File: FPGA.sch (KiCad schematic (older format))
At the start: 1 part

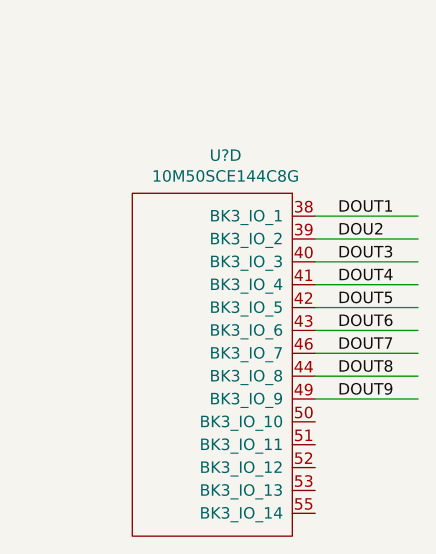
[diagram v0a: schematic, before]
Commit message: sync
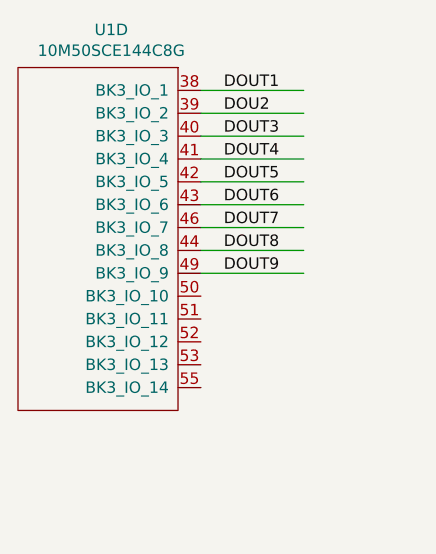
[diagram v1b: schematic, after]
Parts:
- gave numbers to parts that had none: 1
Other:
- moved on the sheet: U1D
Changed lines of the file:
@@
 $EndDescr
 $Comp
-L 10M50SCE:10M50SCE144C8G U?
+L 10M50SCE:10M50SCE144C8G U1
 U 4 1 607B5417
-P 2250 2750
-F 0 "U?" H 1942 3215 50  0000 C CNN
-F 1 "10M50SCE144C8G" H 1942 3124 50  0000 C CNN
-F 2 "10M50SCE144:QFP50P2200X2200X165-145N" H 2250 2750 50  0001 C CNN
-F 3 "" H 2250 2750 50  0001 C CNN
-	4    2250 2750
+P 1750 2200
+F 0 "U1" H 1442 2665 50  0000 C CNN
+F 1 "10M50SCE144C8G" H 1442 2574 50  0000 C CNN
+F 2 "10M50SCE144:QFP50P2200X2200X165-145N" H 1750 2200 50  0001 C CNN
+F 3 "" H 1750 2200 50  0001 C CNN
+	4    1750 2200
 	-1   0    0    -1
 $EndComp
 Wire Wire Line
-	2950 2550 3400 2550
+	2450 2000 2900 2000
 Wire Wire Line
-	2950 2650 3400 2650
+	2450 2100 2900 2100
 Wire Wire Line
-	2950 2750 3400 2750
+	2450 2200 2900 2200
 Wire Wire Line
-	2950 2850 3400 2850
+	2450 2300 2900 2300
 Wire Wire Line
-	2950 2950 3400 2950
+	2450 2400 2900 2400
 Wire Wire Line
-	2950 3050 3400 3050
+	2450 2500 2900 2500
 Wire Wire Line
-	2950 3150 3400 3150
+	2450 2600 2900 2600
 Wire Wire Line
-	2950 3250 3400 3250
+	2450 2700 2900 2700
 Wire Wire Line
-	2950 3350 3400 3350
-Text Label 3050 2550 0    50   ~ 0
+	2450 2800 2900 2800
+Text Label 2550 2000 0    50   ~ 0
 DOUT1
-Text Label 3050 2650 0    50   ~ 0
+Text Label 2550 2100 0    50   ~ 0
 DOU2
-Text Label 3050 2750 0    50   ~ 0
+Text Label 2550 2200 0    50   ~ 0
 DOUT3
-Text Label 3050 2850 0    50   ~ 0
+Text Label 2550 2300 0    50   ~ 0
 DOUT4
-Text Label 3050 2950 0    50   ~ 0
+Text Label 2550 2400 0    50   ~ 0
 DOUT5
-Text Label 3050 3050 0    50   ~ 0
+Text Label 2550 2500 0    50   ~ 0
 DOUT6
-Text Label 3050 3150 0    50   ~ 0
+Text Label 2550 2600 0    50   ~ 0
 DOUT7
-Text Label 3050 3250 0    50   ~ 0
+Text Label 2550 2700 0    50   ~ 0
 DOUT8
-Text Label 3050 3350 0    50   ~ 0
+Text Label 2550 2800 0    50   ~ 0
 DOUT9
 $EndSCHEMATC
